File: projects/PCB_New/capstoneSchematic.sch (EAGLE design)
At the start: 55 parts, among them J1 10118192-0001LF, J2 FTSH-107-01-L-DV-K-A, U1 STM32L476VCT6, U2 LD39050PU33R, U3 74LVC125APW,118, Y1 ABLS-8.000MHZ-B2-T, Y2 ECS-.327-12.5-12QS-TR

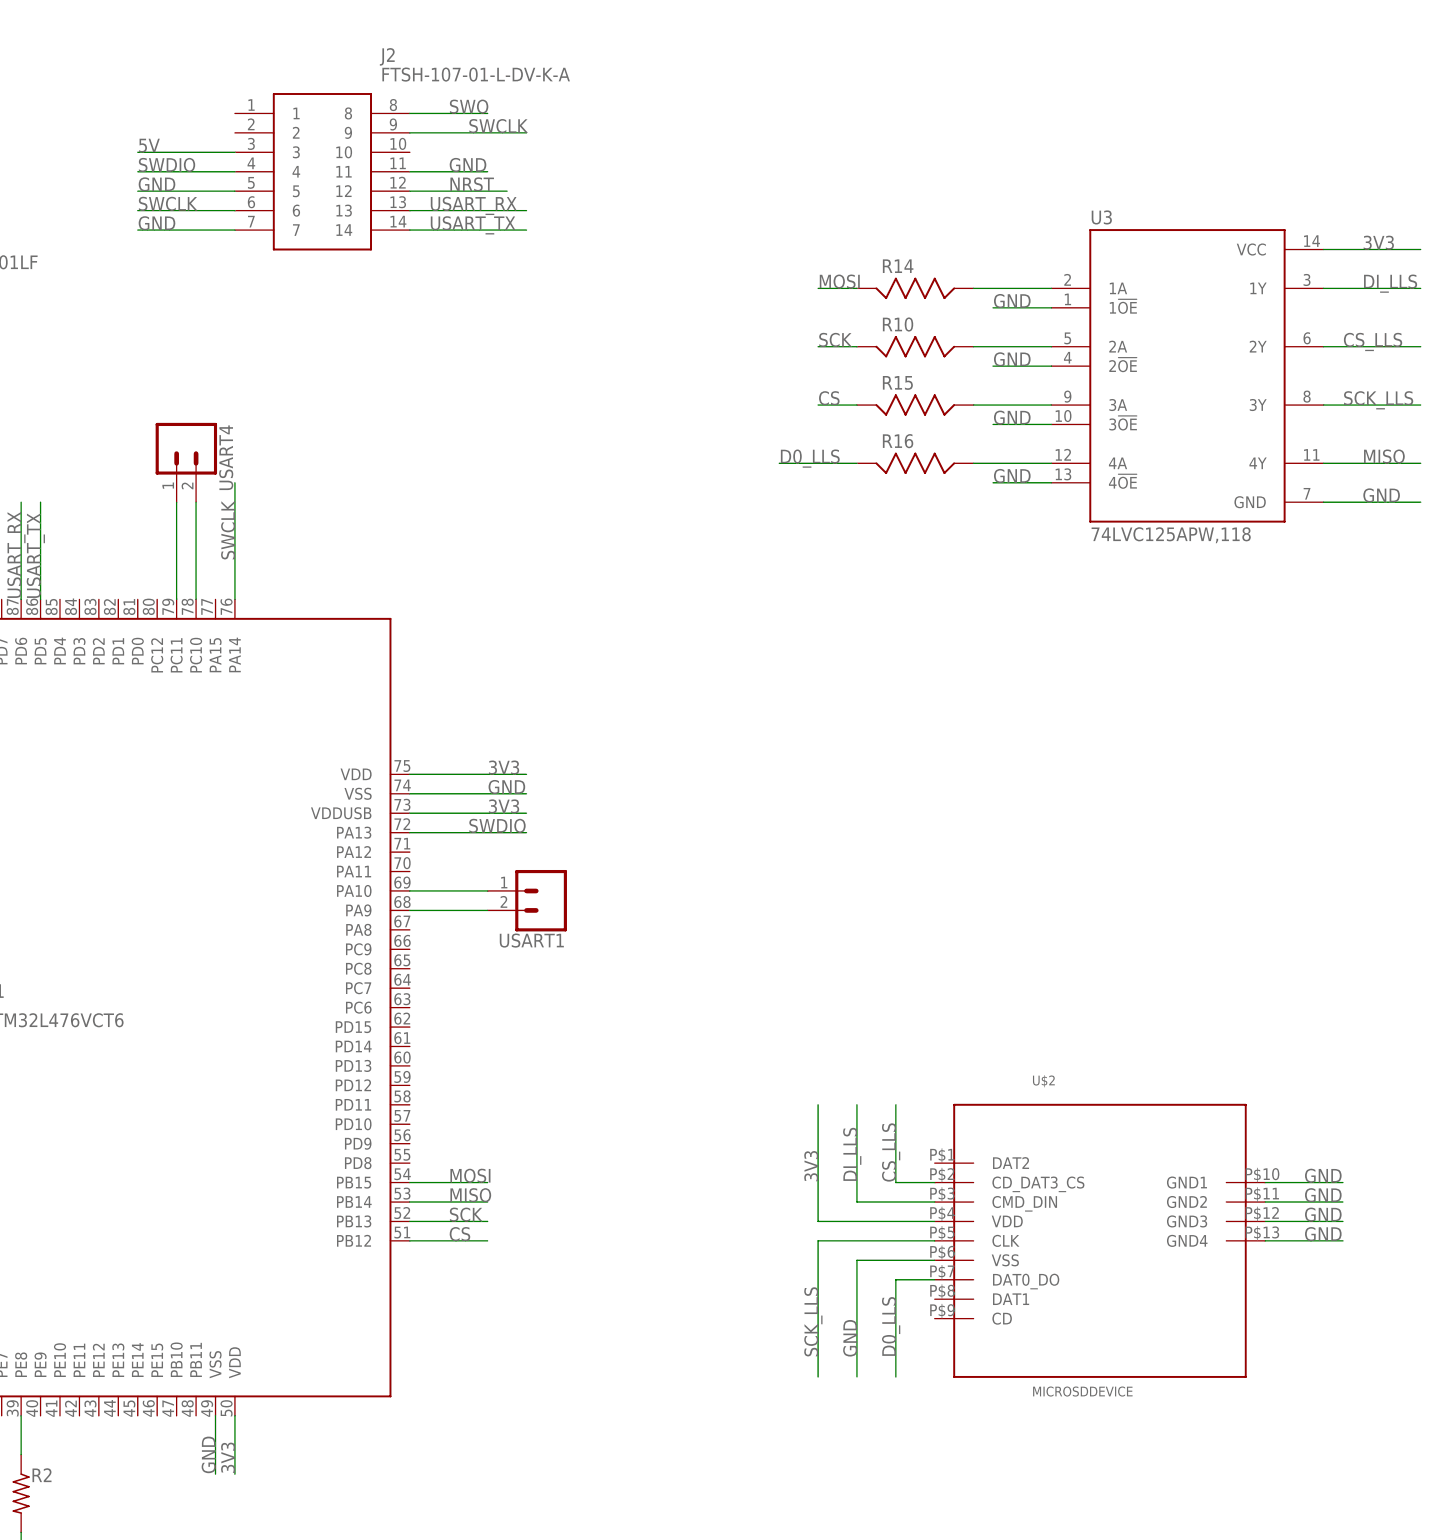
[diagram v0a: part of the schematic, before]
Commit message: V2 Changes
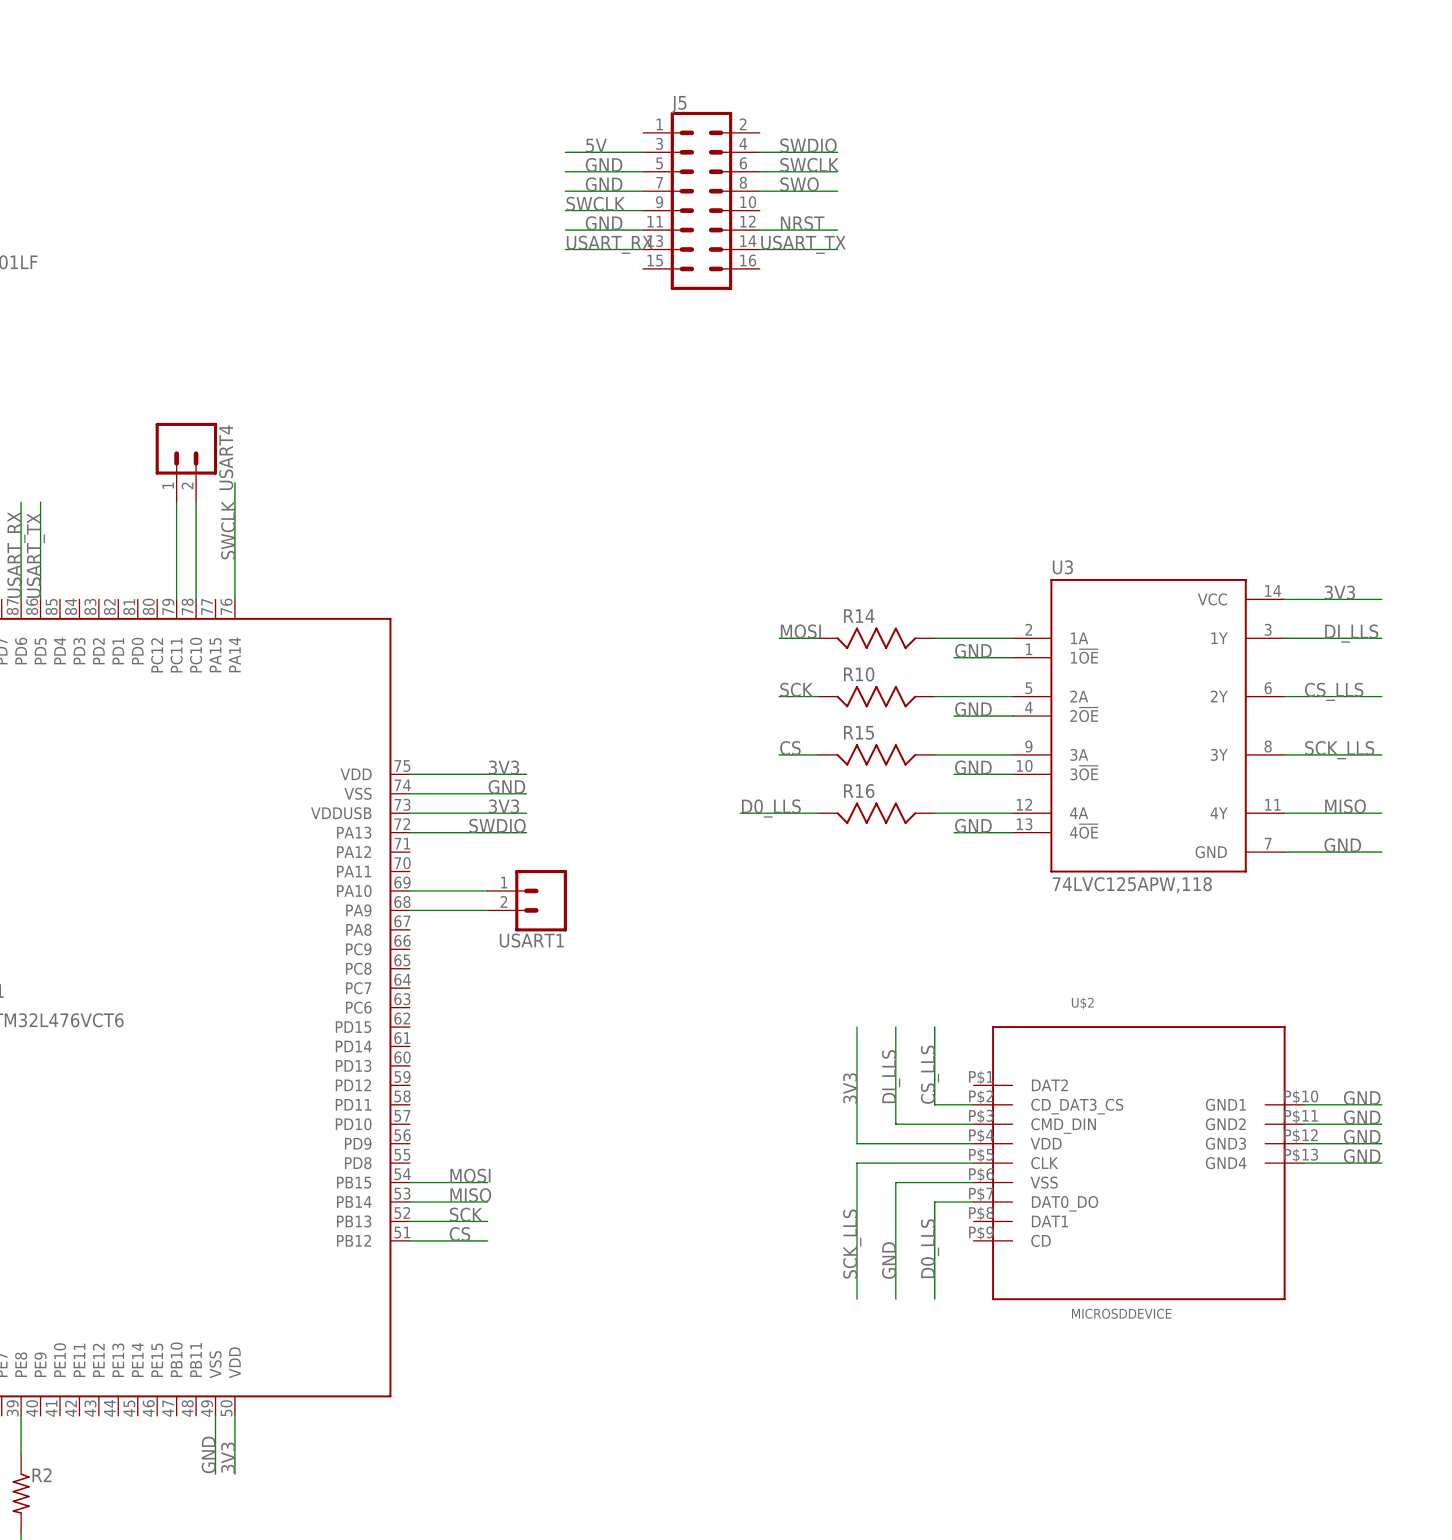
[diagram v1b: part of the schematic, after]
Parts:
- removed J2: FTSH-107-01-L-DV-K-A, ce-capstone:FTSH-107-01-L-DV-K-A
- added J5: (no value), SparkFun-Connectors:CONN_08X2_HEADER
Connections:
- net 5V: now also J5.3; no longer J2.3
- net GND: now also J5.11, J5.5, J5.7; no longer J2.11, J2.5, J2.7
- net NRST: now also J5.12; no longer J2.12
- net SWCLK: now also J5.6, J5.9; no longer J2.6, J2.9
- net SWDIO: now also J5.4; no longer J2.4
- net SWO: now also J5.8; no longer J2.8
- net USART_RX: now also J5.13; no longer J2.13
- net USART_TX: now also J5.14; no longer J2.14
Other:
- moved on the sheet: R10, R14, R15, R16, U$2, U3

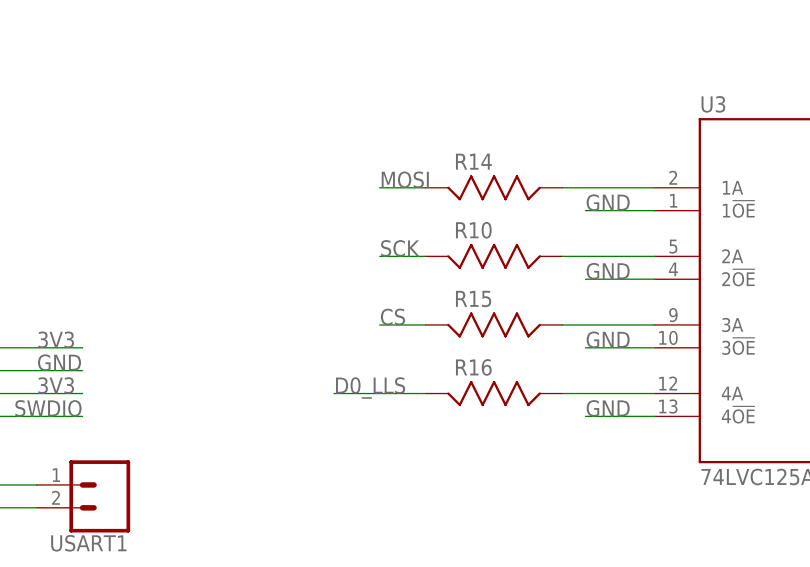
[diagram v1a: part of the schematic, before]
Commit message: SD Changes
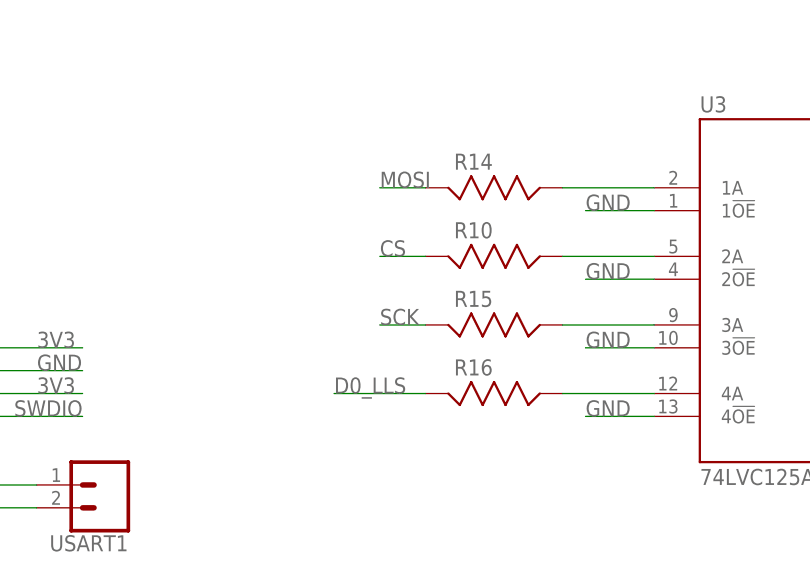
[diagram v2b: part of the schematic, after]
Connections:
- net CS: now also R10.1; no longer R15.1
- net SCK: now also R15.1; no longer R10.1
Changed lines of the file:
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@@
 </segment>
 <segment>
-<pinref part="R10" gate="G$1" pin="1"/>
-<wire x1="170.18" y1="83.82" x2="165.1" y2="83.82" width="0.1524" layer="91"/>
-<label x="165.1" y="83.82" size="1.778" layer="95"/>
+<pinref part="R15" gate="G$1" pin="1"/>
+<wire x1="170.18" y1="76.2" x2="165.1" y2="76.2" width="0.1524" layer="91"/>
+<label x="165.1" y="76.2" size="1.778" layer="95"/>
 </segment>
 </net>
@@
 </segment>
 <segment>
-<pinref part="R15" gate="G$1" pin="1"/>
-<wire x1="170.18" y1="76.2" x2="165.1" y2="76.2" width="0.1524" layer="91"/>
-<label x="165.1" y="76.2" size="1.778" layer="95"/>
+<pinref part="R10" gate="G$1" pin="1"/>
+<wire x1="170.18" y1="83.82" x2="165.1" y2="83.82" width="0.1524" layer="91"/>
+<label x="165.1" y="83.82" size="1.778" layer="95"/>
 </segment>
 </net>

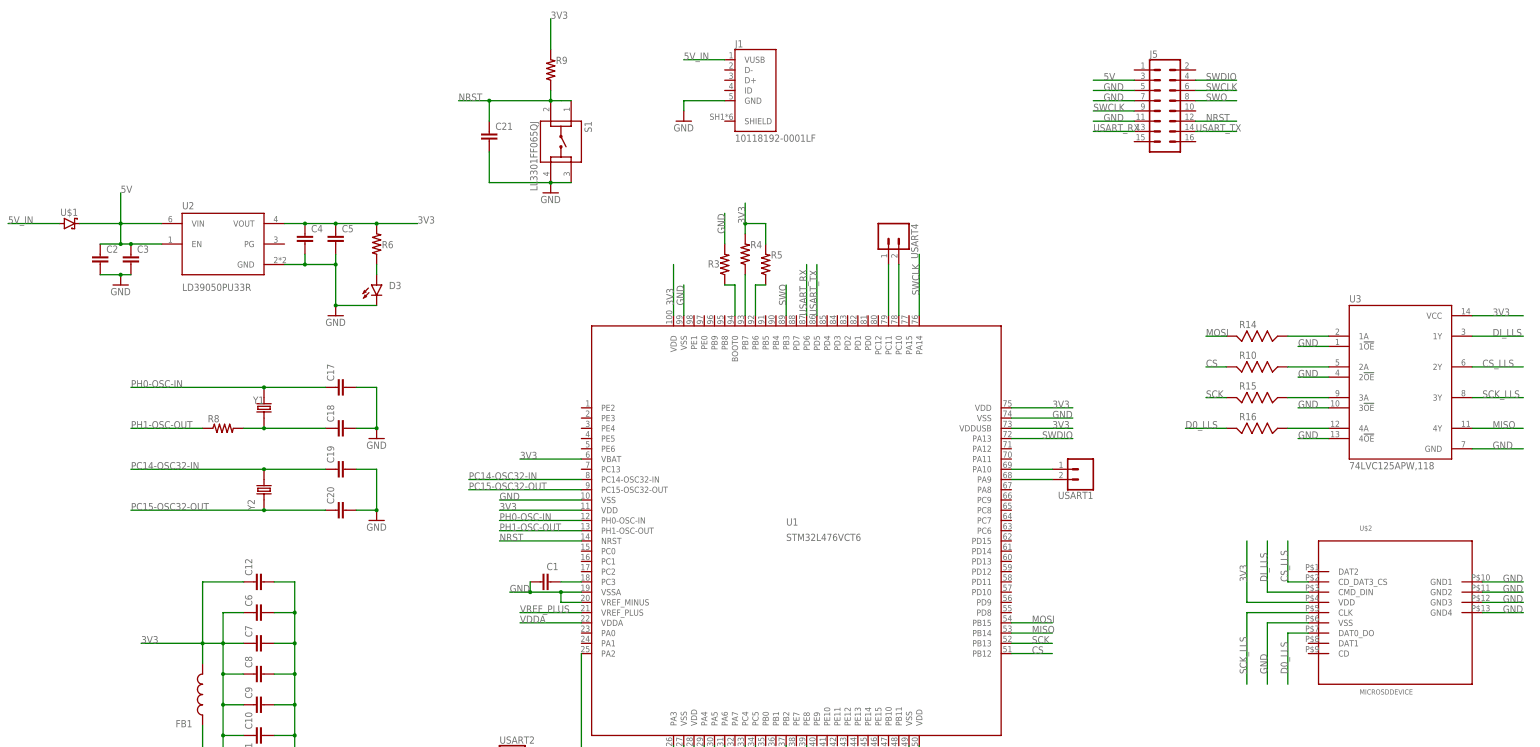
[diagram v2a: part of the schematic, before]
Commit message: SD Buffer Changes
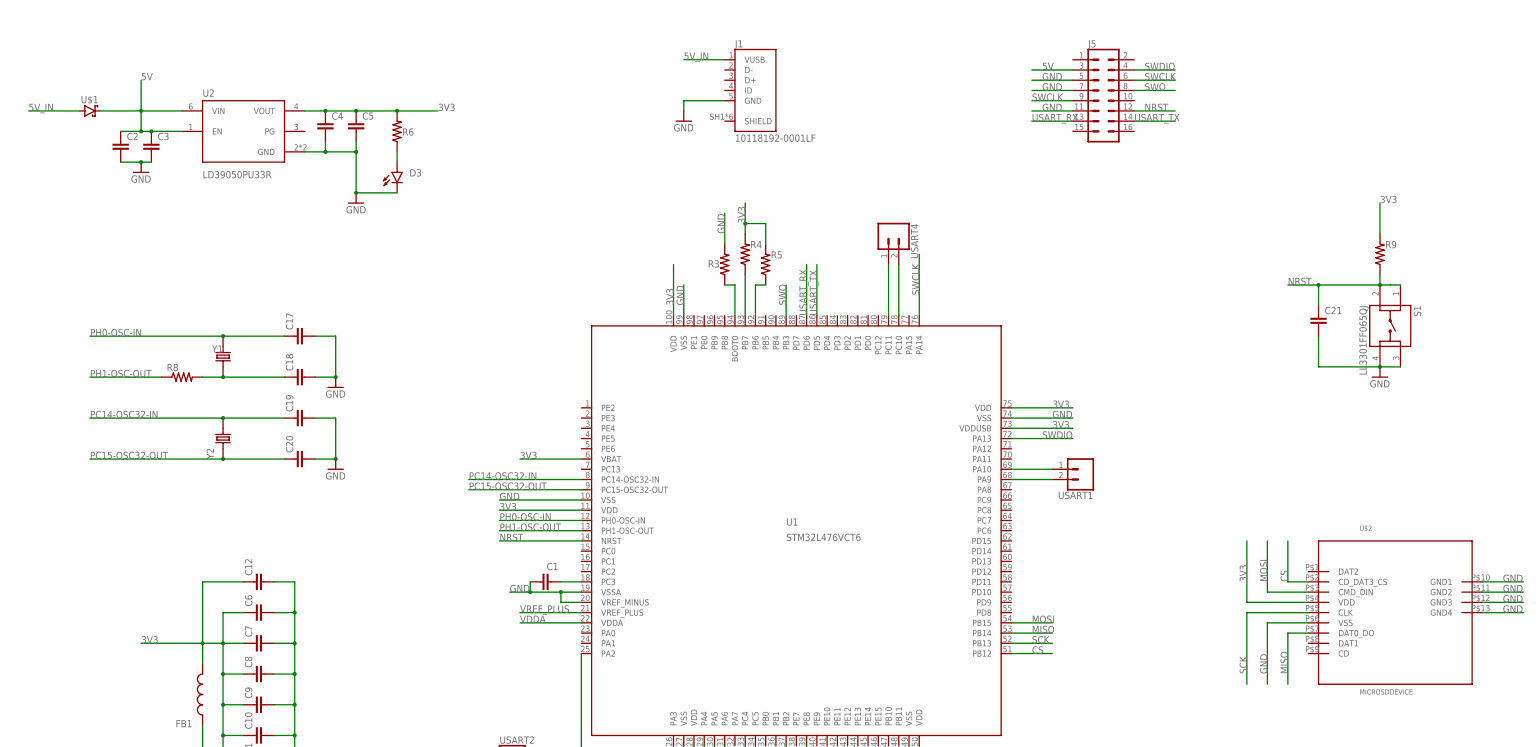
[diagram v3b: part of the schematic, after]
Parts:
- removed R10, R14, R15, R16: RC0402FR-073K3L, RC0402FR-073K3L:RC0402FR-073K3L
- removed U3: 74LVC125APW,118, 74LVC125APW_118:74LVC125APW,118
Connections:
- removed net CS_LLS: U$2.CD_DAT3_CS, U3.2Y
- removed net D0_LLS: R16.1, U$2.DAT0_DO
- removed net DI_LLS: U$2.CMD_DIN, U3.1Y
- removed net N$13: R14.2, U3.1A
- removed net N$24: R10.2, U3.2A
- removed net N$25: R15.2, U3.3A
- removed net N$26: R16.2, U3.4A
- removed net SCK_LLS: U$2.CLK, U3.3Y
- net 3V3: no longer U3.VCC
- net CS: now also U$2.CD_DAT3_CS; no longer R10.1
- net GND: no longer U3.1!OE, U3.2!OE, U3.3!OE, U3.4!OE, U3.GND
- net MISO: now also U$2.DAT0_DO; no longer U3.4Y
- net MOSI: now also U$2.CMD_DIN; no longer R14.1
- net SCK: now also U$2.CLK; no longer R15.1
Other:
- moved on the sheet: C17, C18, C19, C2, C20, C21, C3, C4, C5, D3, J5, R6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
